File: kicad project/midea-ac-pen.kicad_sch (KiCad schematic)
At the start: 8 parts, among them J1 Conn_01x04_Pin, Q1 2N3904, Q2 2N3904

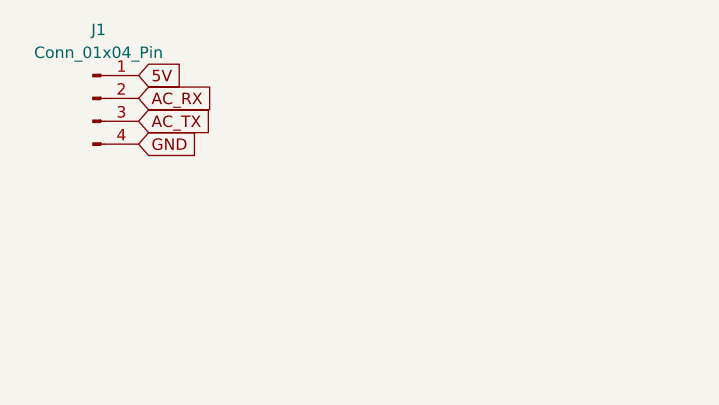
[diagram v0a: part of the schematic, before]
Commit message: Finish board design
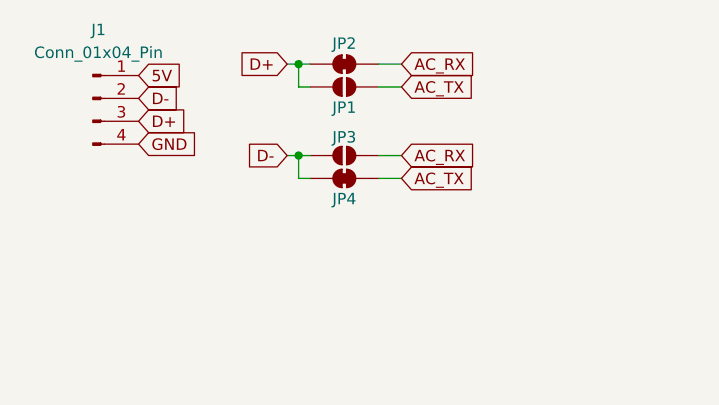
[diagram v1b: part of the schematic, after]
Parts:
- added JP1, JP3: SolderJumper_2_Open, Jumper:SolderJumper-2_P1.3mm_Open_RoundedPad1.0x1.5mm, symbol Jumper:SolderJumper_2_Open
- added JP2, JP4: SolderJumper_2_Bridged, Jumper:SolderJumper-2_P1.3mm_Bridged_RoundedPad1.0x1.5mm, symbol Jumper:SolderJumper_2_Bridged
- U1: value (none) -> ~
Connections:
- net AC_RX: now also JP2.2 (B), JP3.1 (A); no longer J1.2 (Pin_2)
- net AC_TX: now also JP1.1 (A), JP4.2 (B); no longer J1.3 (Pin_3)
- new net D+: J1.3 (Pin_3), JP1.2 (B), JP2.1 (A)
- new net D-: J1.2 (Pin_2), JP3.2 (B), JP4.1 (A)
